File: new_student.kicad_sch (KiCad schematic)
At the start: 39 parts, among them IC1 NCV7351D1ER2G, IC2 TA78L05F_F_, IC3 TA78L05F_F_, J1 RJ45_LED_Shielded, J10 Conn_01x04_Pin, J11 Conn_01x04_Pin, J12 Conn_01x04_Pin, J13 Conn_01x02_Pin, J14 Conn_01x02_Pin, J15 Conn_01x02_Pin, J16 Conn_01x02_Pin, J17 Conn_01x02_Pin, J18 Conn_01x02_Pin, J19 Conn_01x02_Pin, J2 RJ45_LED_Shielded, J20 Conn_01x02_Pin, J3 Conn_01x03_Pin, J4 Conn_01x03_Pin, J5 Conn_01x03_Pin, J6 Conn_01x02_Pin, J7 Conn_01x04_Pin, J8 Conn_01x04_Pin, J9 Conn_01x04_Pin

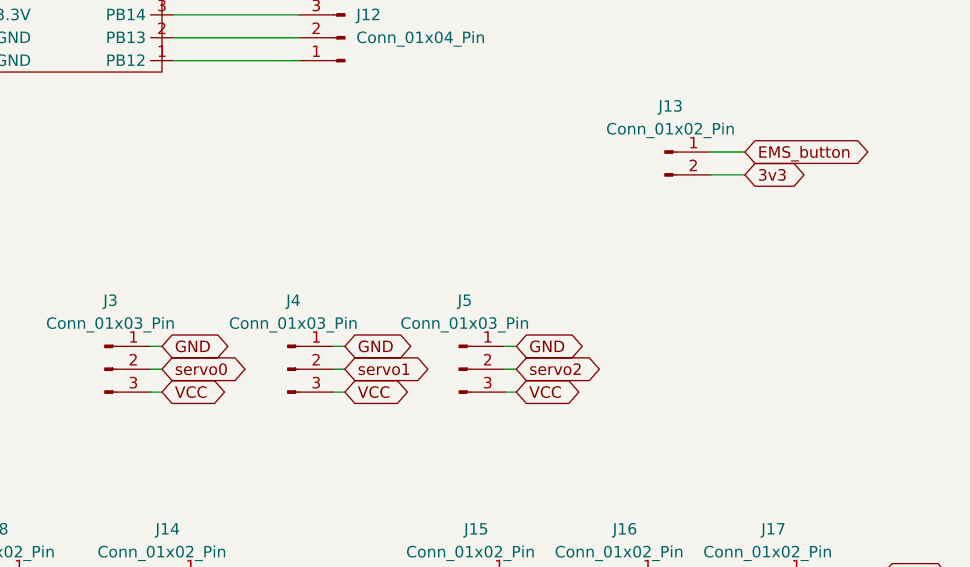
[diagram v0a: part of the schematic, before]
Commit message: Add files via upload
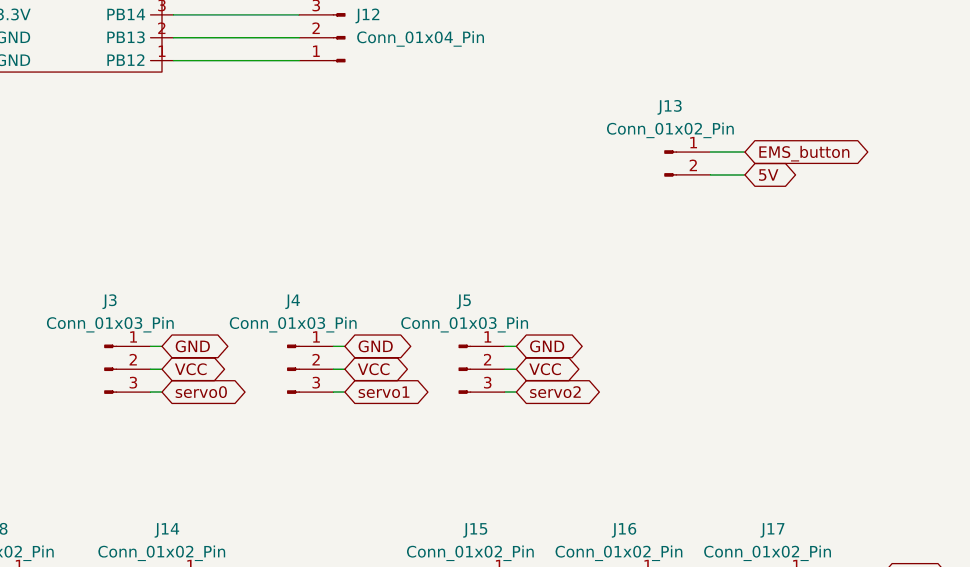
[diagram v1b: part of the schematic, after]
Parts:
- J9: footprint Connector_PinHeader_2.54mm:PinHeader_1x04_P2.54mm_Vertical -> Library:encoder_connect
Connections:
- net 3v3: no longer J13.2 (Pin_2)
- net 5V: now also J13.2 (Pin_2)
- net VCC: now also J3.2 (Pin_2), J4.2 (Pin_2), J5.2 (Pin_2); no longer J3.3 (Pin_3), J4.3 (Pin_3), J5.3 (Pin_3)
- net servo0: now also J3.3 (Pin_3); no longer J3.2 (Pin_2)
- net servo1: now also J4.3 (Pin_3); no longer J4.2 (Pin_2)
- net servo2: now also J5.3 (Pin_3); no longer J5.2 (Pin_2)
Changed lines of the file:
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@@
     )
   )
-  (global_label "VCC" (shape bidirectional) (at 337.82 309.88 0) (fields_autoplaced)
-    (effects (font (size 1.27 1.27)) (justify left))
-    (property "Intersheetrefs" "${INTERSHEET_REFS}" (at 345.5451 309.88 0)
+  (global_label "VCC" (shape bidirectional) (at 337.82 307.34 0) (fields_autoplaced)
+    (effects (font (size 1.27 1.27)) (justify left))
+    (property "Intersheetrefs" "${INTERSHEET_REFS}" (at 345.5451 307.34 0)
       (effects (font (size 1.27 1.27)) (justify left) hide)
     )
@@
     )
   )
-  (global_label "servo0" (shape bidirectional) (at 317.5 307.34 0) (fields_autoplaced)
-    (effects (font (size 1.27 1.27)) (justify left))
-    (property "Intersheetrefs" "${INTERSHEET_REFS}" (at 327.8255 307.34 0)
+  (global_label "servo0" (shape bidirectional) (at 317.5 309.88 0) (fields_autoplaced)
+    (effects (font (size 1.27 1.27)) (justify left))
+    (property "Intersheetrefs" "${INTERSHEET_REFS}" (at 327.8255 309.88 0)
       (effects (font (size 1.27 1.27)) (justify left) hide)
     )
@@
     )
   )
-  (global_label "servo1" (shape bidirectional) (at 337.82 307.34 0) (fields_autoplaced)
-    (effects (font (size 1.27 1.27)) (justify left))
-    (property "Intersheetrefs" "${INTERSHEET_REFS}" (at 348.1455 307.34 0)
+  (global_label "servo1" (shape bidirectional) (at 337.82 309.88 0) (fields_autoplaced)
+    (effects (font (size 1.27 1.27)) (justify left))
+    (property "Intersheetrefs" "${INTERSHEET_REFS}" (at 348.1455 309.88 0)
       (effects (font (size 1.27 1.27)) (justify left) hide)
     )
@@
     )
   )
-  (global_label "servo2" (shape bidirectional) (at 356.87 307.34 0) (fields_autoplaced)
-    (effects (font (size 1.27 1.27)) (justify left))
-    (property "Intersheetrefs" "${INTERSHEET_REFS}" (at 367.1955 307.34 0)
+  (global_label "servo2" (shape bidirectional) (at 356.87 309.88 0) (fields_autoplaced)
+    (effects (font (size 1.27 1.27)) (justify left))
+    (property "Intersheetrefs" "${INTERSHEET_REFS}" (at 367.1955 309.88 0)
       (effects (font (size 1.27 1.27)) (justify left) hide)
     )
@@
     )
   )
-  (global_label "VCC" (shape bidirectional) (at 317.5 309.88 0) (fields_autoplaced)
-    (effects (font (size 1.27 1.27)) (justify left))
-    (property "Intersheetrefs" "${INTERSHEET_REFS}" (at 325.2251 309.88 0)
+  (global_label "VCC" (shape bidirectional) (at 317.5 307.34 0) (fields_autoplaced)
+    (effects (font (size 1.27 1.27)) (justify left))
+    (property "Intersheetrefs" "${INTERSHEET_REFS}" (at 325.2251 307.34 0)
       (effects (font (size 1.27 1.27)) (justify left) hide)
     )
@@
     )
   )
-  (global_label "VCC" (shape bidirectional) (at 356.87 309.88 0) (fields_autoplaced)
-    (effects (font (size 1.27 1.27)) (justify left))
-    (property "Intersheetrefs" "${INTERSHEET_REFS}" (at 364.5951 309.88 0)
+  (global_label "VCC" (shape bidirectional) (at 356.87 307.34 0) (fields_autoplaced)
+    (effects (font (size 1.27 1.27)) (justify left))
+    (property "Intersheetrefs" "${INTERSHEET_REFS}" (at 364.5951 307.34 0)
       (effects (font (size 1.27 1.27)) (justify left) hide)
     )
@@
     )
   )
-  (global_label "3v3" (shape bidirectional) (at 382.27 285.75 0) (fields_autoplaced)
-    (effects (font (size 1.27 1.27)) (justify left))
-    (property "Intersheetrefs" "${INTERSHEET_REFS}" (at 389.7531 285.75 0)
+  (global_label "5V" (shape bidirectional) (at 382.27 285.75 0) (fields_autoplaced)
+    (effects (font (size 1.27 1.27)) (justify left))
+    (property "Intersheetrefs" "${INTERSHEET_REFS}" (at 388.6646 285.75 0)
       (effects (font (size 1.27 1.27)) (justify left) hide)
     )
@@
       (effects (font (size 1.27 1.27)))
     )
-    (property "Footprint" "Connector_PinHeader_2.54mm:PinHeader_1x04_P2.54mm_Vertical" (at 232.41 236.22 0)
-      (effects (font (size 1.27 1.27)) hide)
-    )
+    (property "Footprint" "Library:encoder_connect" (at 232.41 236.22 0)
+      (effects (font (size 1.27 1.27)) hide)
+    )
